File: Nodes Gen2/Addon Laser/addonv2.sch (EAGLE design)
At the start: 59 parts, among them J3 22-05-7038-03, J4 22-05-7048-04, J5 22-05-7048-04

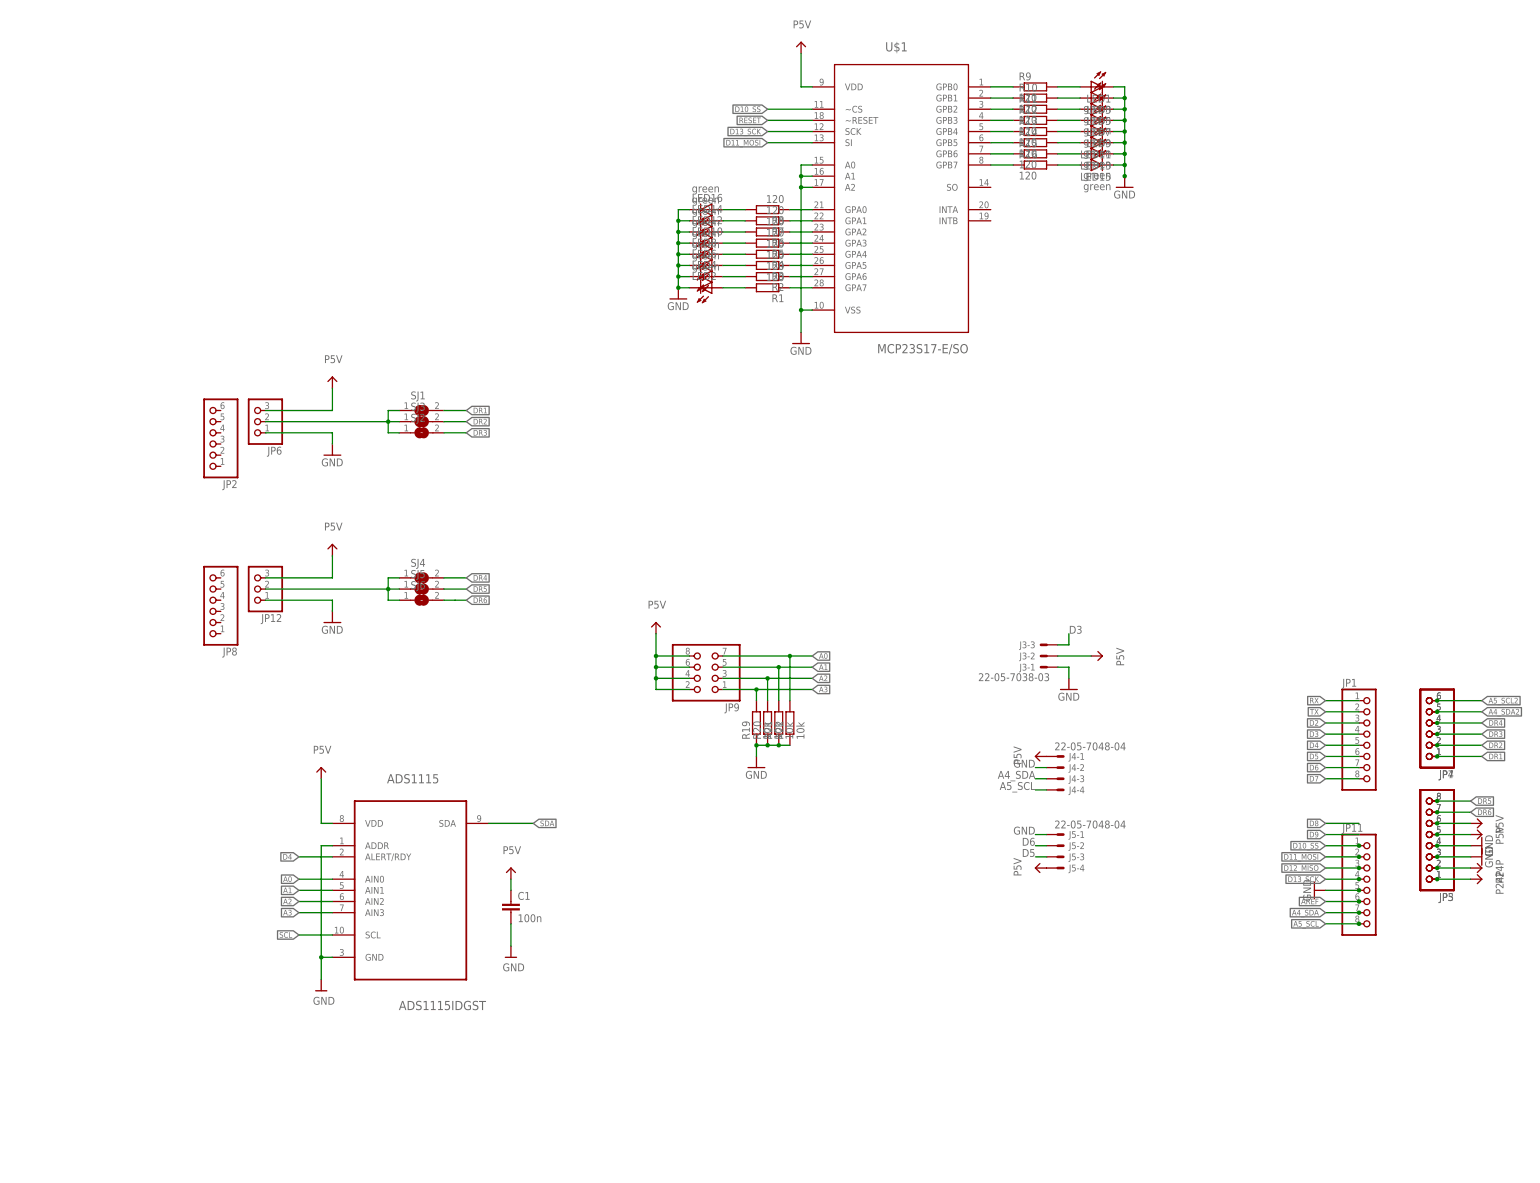
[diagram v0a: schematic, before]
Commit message: gen 2 dev + bom
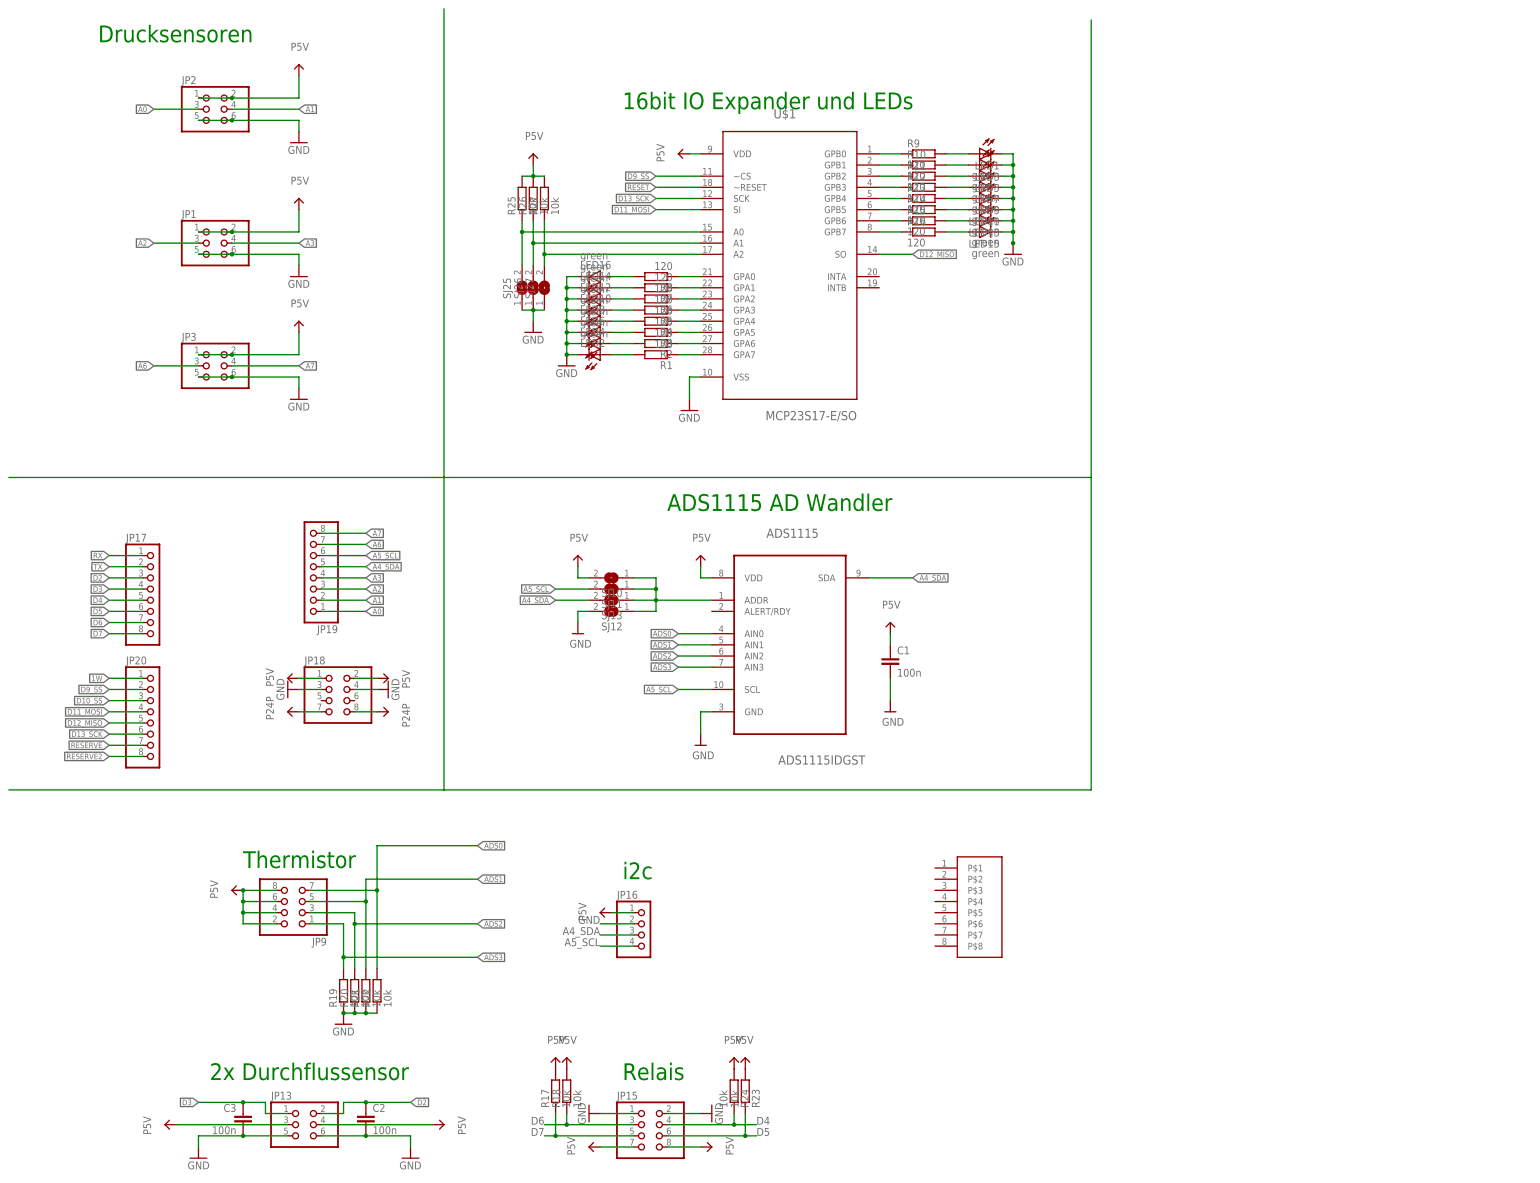
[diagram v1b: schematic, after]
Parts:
- removed J3: 22-05-7038-03, con-molex:22-05-7038-03
- removed J4, J5: 22-05-7048-04, con-molex:22-05-7048-04
- removed JP11, JP5: (no value), pinhead:PINHD-1X8
- removed JP12, JP6: (no value), pinhead:PINHD-1X3
- removed JP4, JP7, JP8: (no value), pinhead:PINHD-1X6
- removed SJ1, SJ2, SJ3, SJ4, SJ5, SJ6: (no value), jumper:SJ
- added C2, C3: 100n, schlager_passiv:C-EUC0805
- added JP13: (no value), pinhead:PINHD-2X3/90
- added JP15: (no value), pinhead:PINHD-2X4/90
- added JP16: (no value), pinhead:PINHD-1X4/90
- added JP17, JP19, JP20: (no value), pinhead:PINHD-1X8
- added JP18: (no value), pinhead:PINHD-2X4
- added R17, R18, R23, R24, R25, R26, R27: 10k, rcl:R-EU_R0805
- added SJ10, SJ11, SJ12, SJ13, SJ25, SJ26, SJ27: (no value), jumper:SJN
- added U$2: 1.44-128X128, schlager_modules:1.44-128X128
- JP1, JP3: device pinhead:PINHD-1X8 -> pinhead:PINHD-2X3/90
- JP2: device pinhead:PINHD-1X6 -> pinhead:PINHD-2X3/90
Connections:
- removed net A4_SDA2: JP4.5, JP7.5
- removed net A5_SCL2: JP4.6, JP7.6
- removed net AREF: JP11.6
- removed net DR1: JP4.1, JP7.1, SJ1.2
- removed net DR2: JP4.2, JP7.2, SJ3.2
- removed net DR3: JP4.3, JP7.3, SJ2.2
- removed net DR4: JP4.4, JP7.4, SJ4.2
- removed net DR5: JP3.8, JP5.8, SJ5.2
- removed net DR6: JP3.7, JP5.7, SJ6.2
- removed net N$33: JP6.2, SJ1.1, SJ2.1, SJ3.1
- removed net N$34: JP12.2, SJ4.1, SJ5.1, SJ6.1
- removed net SCL: ADS1115.SCL
- removed net SDA: ADS1115.SDA
- new net 1W: JP20.1
- new net A6: JP19.7, JP3.3
- new net A7: JP19.8, JP3.4
- new net ADS0: ADS1115.AIN0, JP9.7, R22.2
- new net ADS1: ADS1115.AIN1, JP9.5, R21.2
- new net ADS2: ADS1115.AIN2, JP9.3, R20.2
- new net ADS3: ADS1115.AIN3, JP9.1, R19.2
- new net D9_SS: JP20.2, U$1.~CS
- new net N$36: ADS1115.ADDR, SJ10.1, SJ11.1, SJ12.1, SJ13.1
- new net N$38: R25.1, SJ25.2, U$1.A0
- new net N$39: R26.1, SJ26.2, U$1.A1
- new net N$40: R27.1, SJ27.2, U$1.A2
- new net RESERVE: JP20.7
- new net RESERVE2: JP20.8
- net A0: now also JP19.1, JP2.3; no longer ADS1115.AIN0, JP9.7, R22.2
- net A1: now also JP19.2, JP2.4; no longer ADS1115.AIN1, JP9.5, R21.2
- net A2: now also JP1.3, JP19.3; no longer ADS1115.AIN2, JP9.3, R20.2
- net A3: now also JP1.4, JP19.4; no longer ADS1115.AIN3, JP9.1, R19.2
- net A4_SDA: now also ADS1115.SDA, JP16.3, JP19.5, SJ13.2; no longer J4-3.S, JP11.7
- net A5_SCL: now also ADS1115.SCL, JP16.4, JP19.6, SJ11.2; no longer J4-4.S, JP11.8
- net D10_SS: now also JP20.3; no longer JP11.1, U$1.~CS
- net D11_MOSI: now also JP20.4; no longer JP11.2
- net D12_MISO: now also JP20.5, U$1.SO; no longer JP11.3
- net D13_SCK: now also JP20.6; no longer JP11.4
- net D2: now also C2.1, JP13.2, JP17.3; no longer JP1.3
- net D3: now also C3.1, JP13.1, JP17.4; no longer J3-3.S, JP1.4
- net D4: now also JP15.4, JP17.5, R24.1; no longer ADS1115.ALERT/RDY, JP1.5
- net D5: now also JP15.6, JP17.6, R23.1; no longer J5-3.S, JP1.6
- net D6: now also JP15.3, JP17.7, R18.1; no longer J5-2.S, JP1.7
- net D7: now also JP15.5, JP17.8, R17.1; no longer JP1.8
- net GND: now also C2.2, C3.2, JP1.5, JP1.6, JP13.5, JP13.6, JP15.1, JP15.2, JP16.2, JP18.3, JP18.4, JP2.5, JP2.6, JP3.5, JP3.6, SJ12.2, SJ25.1, SJ26.1, SJ27.1; no longer ADS1115.ADDR, J3-1.S, J4-2.S, J5-1.S, JP11.5, JP12.1, JP3.3, JP3.4, JP5.3, JP5.4, JP6.1, U$1.A0, U$1.A1, U$1.A2
- net P24P: now also JP18.7, JP18.8; no longer JP3.1, JP3.2, JP5.1, JP5.2
- net P5V: now also JP1.1, JP1.2, JP13.3, JP13.4, JP15.7, JP15.8, JP16.1, JP18.1, JP18.2, JP2.1, JP2.2, JP3.1, JP3.2, R17.2, R18.2, R23.2, R24.2, R25.2, R26.2, R27.2, SJ10.2; no longer J3-2.S, J4-1.S, J5-4.S, JP12.3, JP3.5, JP3.6, JP5.5, JP5.6, JP6.3
- net RX: now also JP17.1; no longer JP1.1
- net TX: now also JP17.2; no longer JP1.2
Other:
- note added: "16bit IO Expander und LEDs"
- note added: "2x Durchflussensor"
- note added: "ADS1115 AD Wandler"
- note added: "Drucksensoren"
- note added: "Relais"
- note added: "Thermistor"
- note added: "i2c"
- moved on the sheet: ADS1115, C1, JP2, JP9, LED1, LED10, LED11, LED12, LED13, LED14, LED15, LED16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
